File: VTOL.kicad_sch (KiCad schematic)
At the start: 17 parts, among them J1 Conn_01x04_Pin, SW1 RESET, SW2 RESET

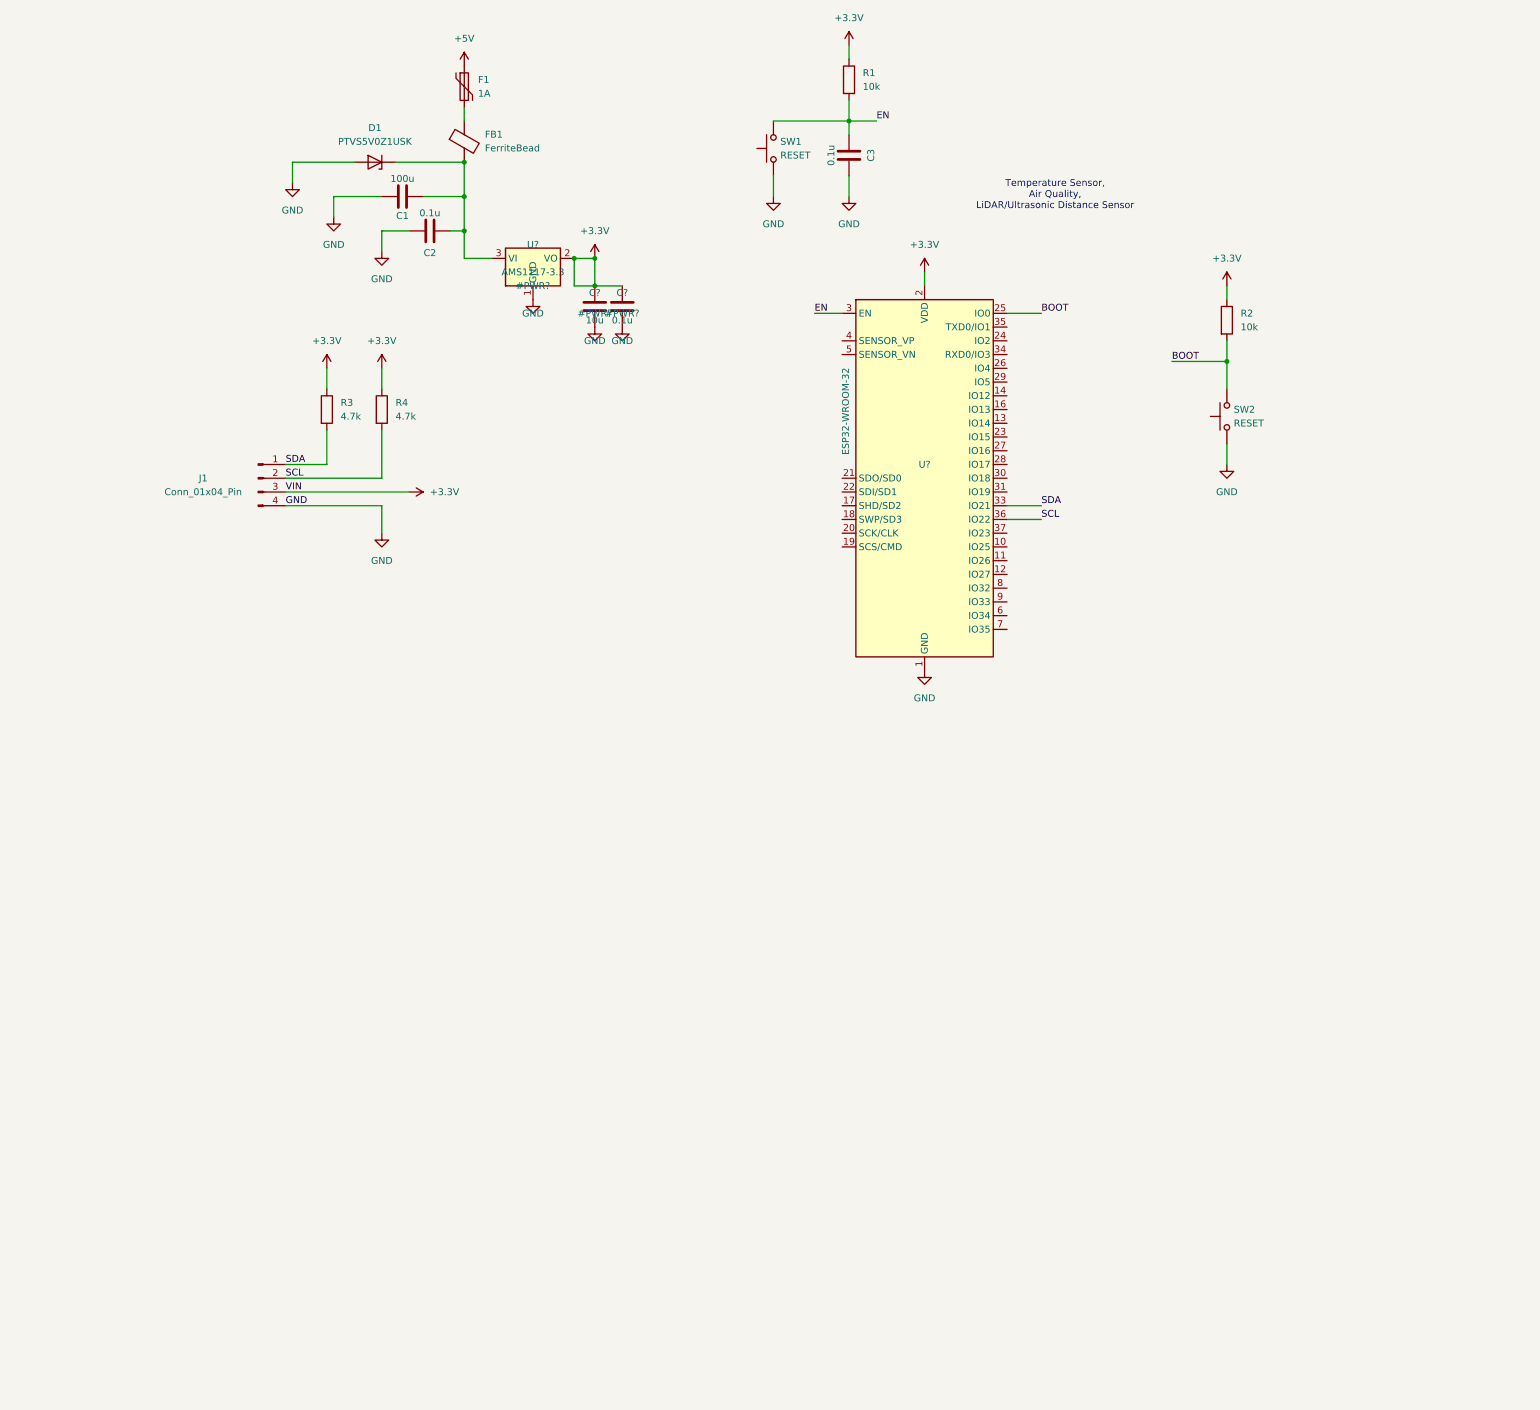
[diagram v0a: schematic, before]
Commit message: finished the schem
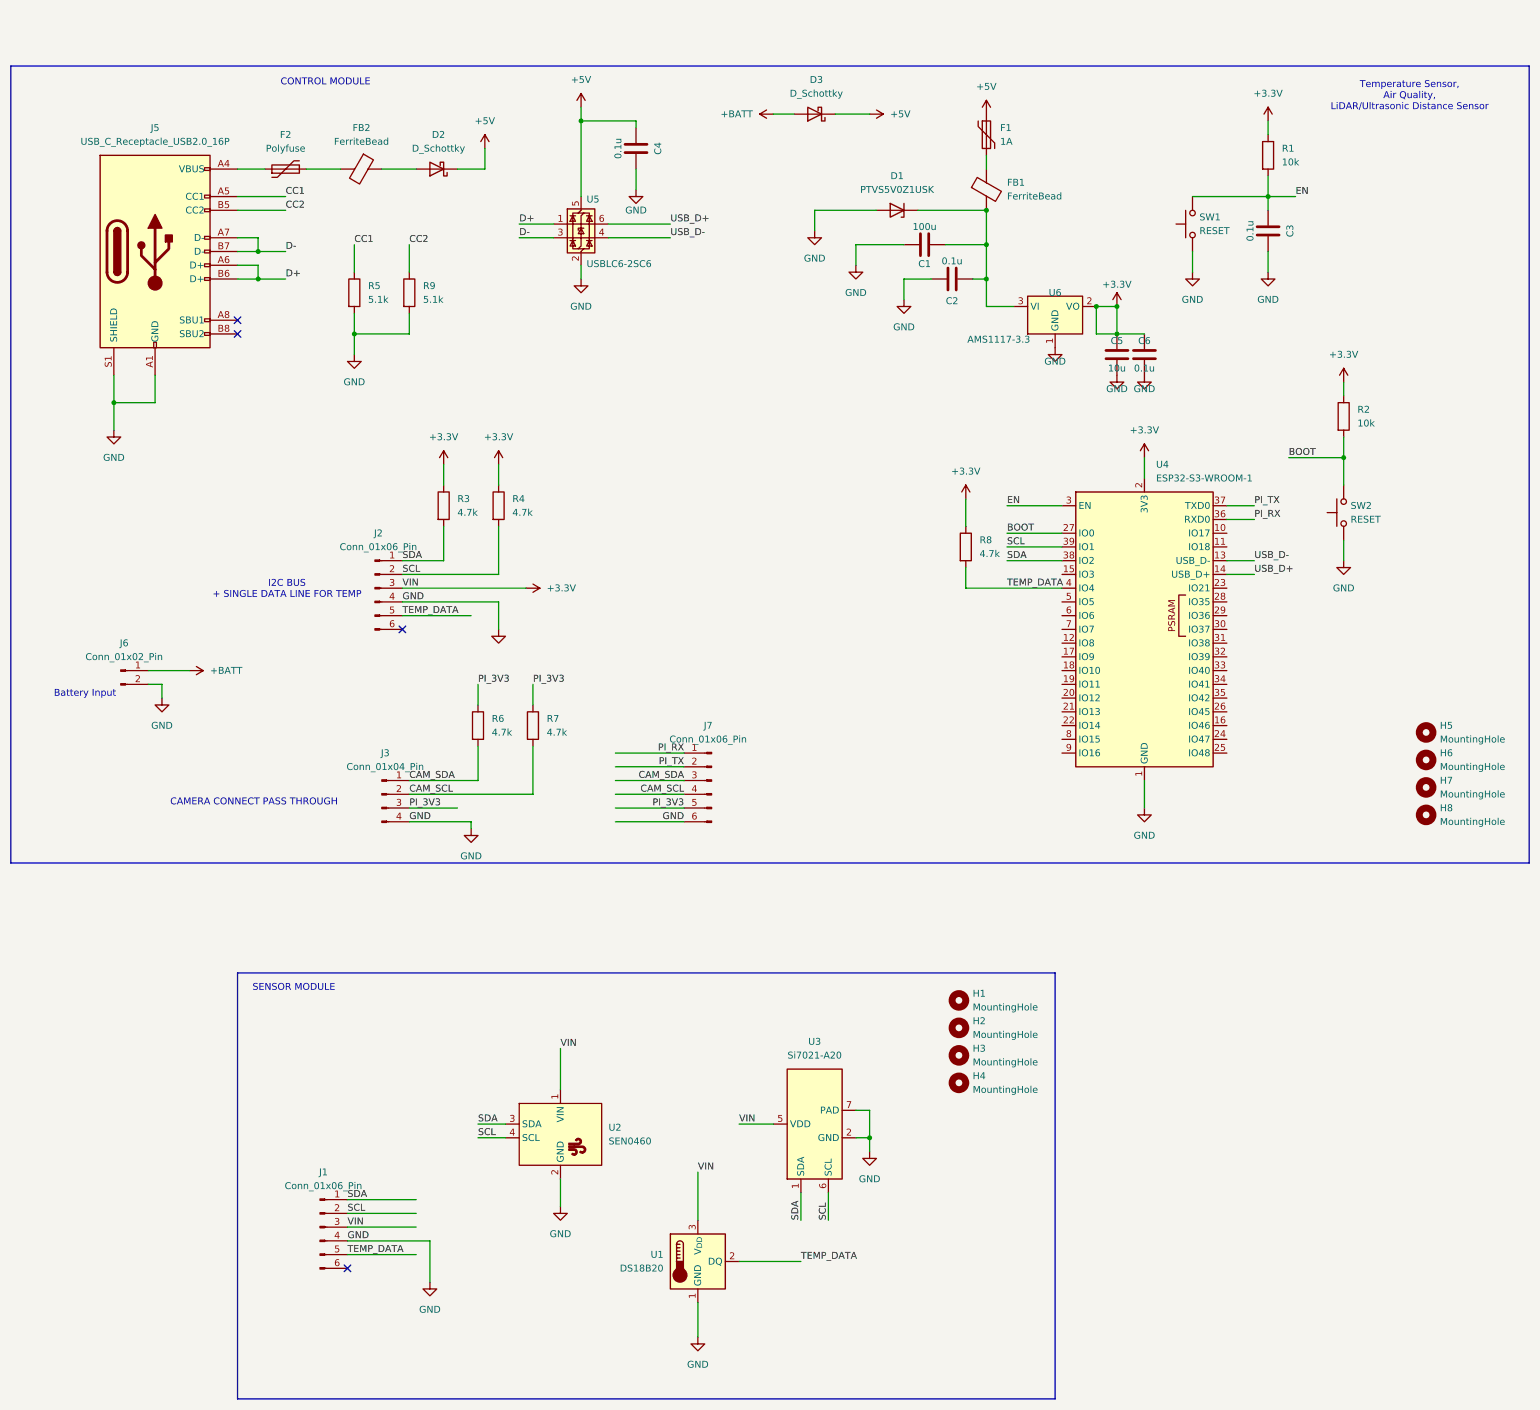
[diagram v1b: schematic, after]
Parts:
- removed J1: Conn_01x04_Pin, symbol Connector:Conn_01x04_Pin
- removed U?: ESP32-WROOM-32, RF_Module:ESP32-WROOM-32, symbol RF_Module:ESP32-WROOM-32
- added C4: 0.1u, symbol Device:C
- added D2, D3: D_Schottky, symbol Device:D_Schottky
- added F2: Polyfuse, symbol Device:Polyfuse
- added FB2: FerriteBead, symbol Device:FerriteBead
- added H1, H2, H3, H4, H5, H6, H7, H8: MountingHole, symbol Mechanical:MountingHole
- added J1, J2, J7: Conn_01x06_Pin, symbol Connector:Conn_01x06_Pin
- added J3: Conn_01x04_Pin, symbol Connector:Conn_01x04_Pin
- added J5: USB_C_Receptacle_USB2.0_16P, symbol Connector:USB_C_Receptacle_USB2.0_16P
- added J6: Conn_01x02_Pin, symbol Connector:Conn_01x02_Pin
- added R5, R9: 5.1k, symbol Device:R
- added R6, R7, R8: 4.7k, symbol Device:R
- added U1: DS18B20, Package_TO_SOT_THT:TO-92_Inline, symbol Sensor_Temperature:DS18B20
- added U2: SEN0460, symbol Sensor_Symbols:SEN0460
- added U3: Si7021-A20, Package_DFN_QFN:DFN-6-1EP_3x3mm_P1mm_EP1.5x2.4mm, symbol Sensor_Humidity:Si7021-A20
- added U4: ESP32-S3-WROOM-1, RF_Module:ESP32-S3-WROOM-1, symbol RF_Module:ESP32-S3-WROOM-1
- added U5: USBLC6-2SC6, Package_TO_SOT_SMD:SOT-23-6, symbol Power_Protection:USBLC6-2SC6
- gave numbers to parts that had none: 3
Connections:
- net +3.3V: now also J1.3 (Pin_3), J2.3 (Pin_3), R8.1, U1.3 (V_{DD}), U2.1 (VIN), U3.5 (VDD), U4.2 (3V3)
- net +5V: now also C4.2, D2.1 (K), D3.1 (K), U5.5 (VBUS)
- net BOOT: now also U4.27 (IO0)
- net EN: now also U4.3 (EN)
- net GND: now also C4.1, J1.4 (Pin_4), J2.4 (Pin_4), J3.4 (Pin_4), J5.A1 (GND), J5.A12 (GND), J5.B1 (GND), J5.B12 (GND), J5.S1 (SHIELD), J6.2 (Pin_2), J7.6 (Pin_6), R5.2, R9.2, U1.1 (GND), U2.2 (GND), U3.2 (GND), U3.7 (PAD), U4.1 (GND), U4.40 (GND), U4.41 (GND), U5.2 (GND)
- net SCL: now also J1.2 (Pin_2), J2.2 (Pin_2), U2.4 (SCL), U3.6 (SCL), U4.39 (IO1)
- net SDA: now also J1.1 (Pin_1), J2.1 (Pin_1), U2.3 (SDA), U3.1 (SDA), U4.38 (IO2)
- new net: D2.2 (A), FB2.1
- new net: F2.2, FB2.2
- new net: F2.1, J5.A4 (VBUS), J5.A9 (VBUS), J5.B4 (VBUS), J5.B9 (VBUS)
- new net +BATT: D3.2 (A), J6.1 (Pin_1)
- new net CAM_SCL: J3.2 (Pin_2), J7.4 (Pin_4), R7.2
- new net CAM_SDA: J3.1 (Pin_1), J7.3 (Pin_3), R6.2
- new net CC1: J5.A5 (CC1), R5.1
- new net CC2: J5.B5 (CC2), R9.1
- new net D+: J5.A6 (D+), J5.B6 (D+), U5.1 (I/O1)
- new net D-: J5.A7 (D-), J5.B7 (D-), U5.3 (I/O2)
- new net PI_3V3: J3.3 (Pin_3), J7.5 (Pin_5), R6.1, R7.1
- new net PI_RX: J7.1 (Pin_1), U4.36 (RXD0)
- new net PI_TX: J7.2 (Pin_2), U4.37 (TXD0)
- new net TEMP_DATA: J1.5 (Pin_5), J2.5 (Pin_5), R8.2, U1.2 (DQ), U4.4 (IO4)
- new net USB_D+: U4.14 (USB_D+), U5.6 (I/O1)
- new net USB_D-: U4.13 (USB_D-), U5.4 (I/O2)
- no-connect marks 0 -> 4
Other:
- note added: "Battery Input"
- note added: "CAMERA CONNECT PASS THROUGH"
- note added: "CONTROL MODULE"
- note added: "I2C BUS + SINGLE DATA LINE FOR TEMP"
- note added: "SENSOR MODULE"
- moved on the sheet: C1, C2, C3, C5, C6, D1, F1, FB1, R1, R2, R3, R4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
